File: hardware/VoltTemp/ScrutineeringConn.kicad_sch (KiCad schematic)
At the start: 3 parts, among them J1 ScrutineeringConn

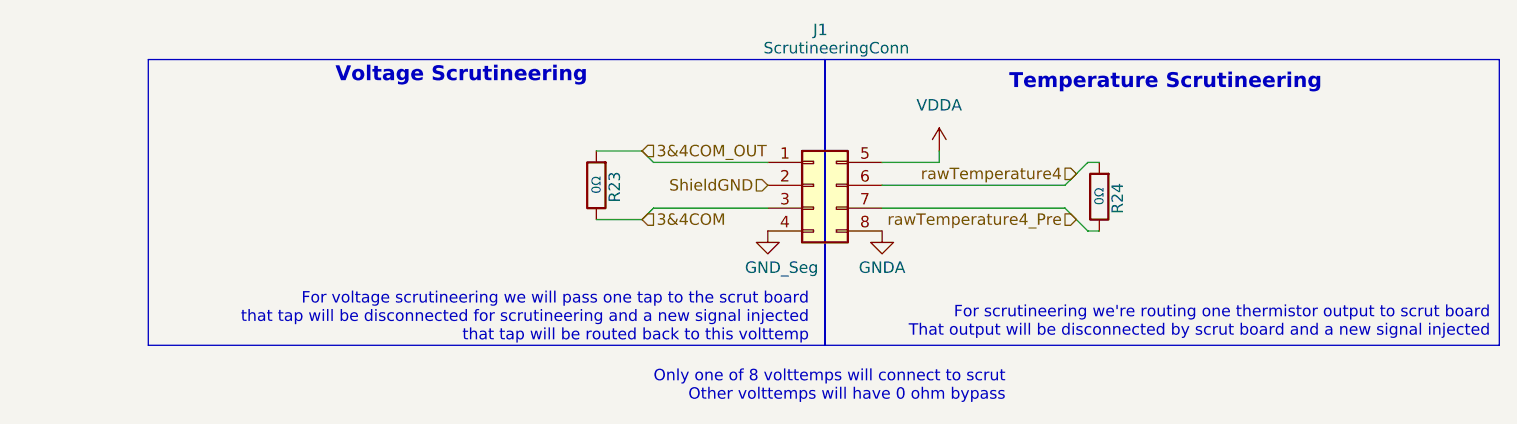
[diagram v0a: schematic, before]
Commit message: bom
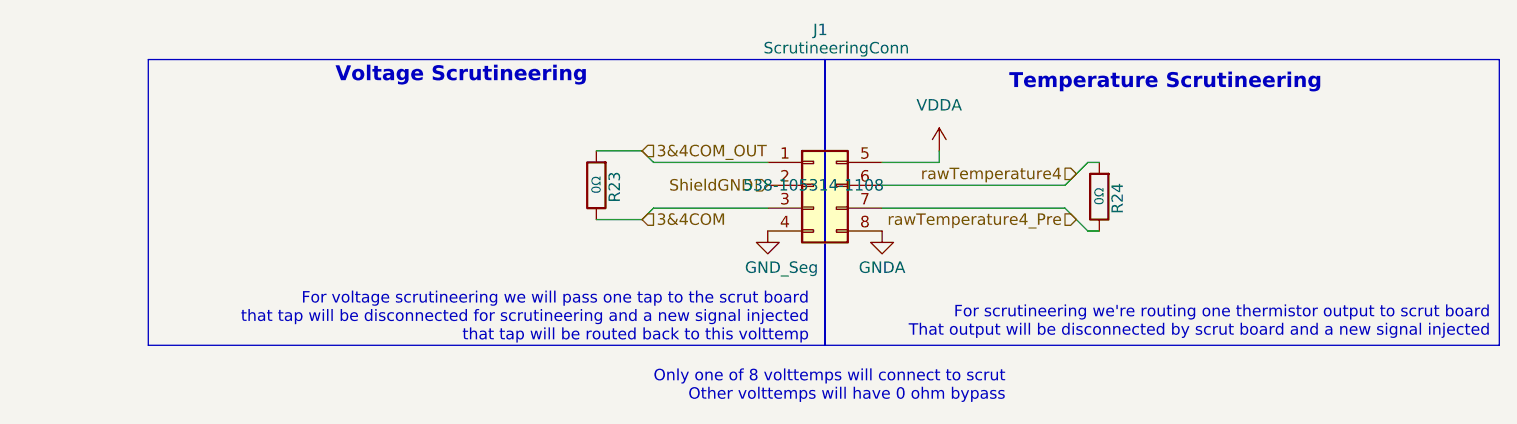
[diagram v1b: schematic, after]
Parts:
- J1: P/N (none) -> 538-105314-1108
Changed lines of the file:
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@@
 			)
 		)
-		(property "Datasheet" "~"
+		(property "Datasheet" "https://tools.molex.com/pdm_docs/sd/1053141108_sd.pdf"
 			(at 90.17 57.15 0)
 			(effects
@@
 			)
 		)
+		(property "P/N" "538-105314-1108"
+			(at 90.17 57.15 0)
+			(effects
+				(font
+					(size 1.27 1.27)
+				)
+			)
+		)
